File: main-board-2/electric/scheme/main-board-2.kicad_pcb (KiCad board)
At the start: 2 copper layers, 85 x 56 mm, 125 parts, among them K1 power-switch, K2 usb-power-switch, P1 batt, P10 rst, P11 screw-1, P13 screw-2, P14 gpio-big, P15 gpio-small, P16 moto-1, P17 moto-2, P2 CONN_4, P3 trigger-btn, P4 CONN_3X2, P5 reg-short-to-gnd-1, P6 reg-short-to-gnd-2, P7 bootloader, P8 cross board conn, P9 rst, Q1 IRLML2244, Q10 IRLML2244, Q11 sot223, Q12 bc857, Q13 irlml2244, Q2 BC847, Q3 IRLML2244, Q4 IRLML2244, Q5 BC847, Q6 BC847, Q7 BC847, Q8 BC847, Q9 IRLML2244, U1 LM317AEMP, U2 LM317AT, U3 LM317AEMP, U4 LM317AT, U5 LM293, U6 L298, U7 MINI-USB-B, X1 8MHz

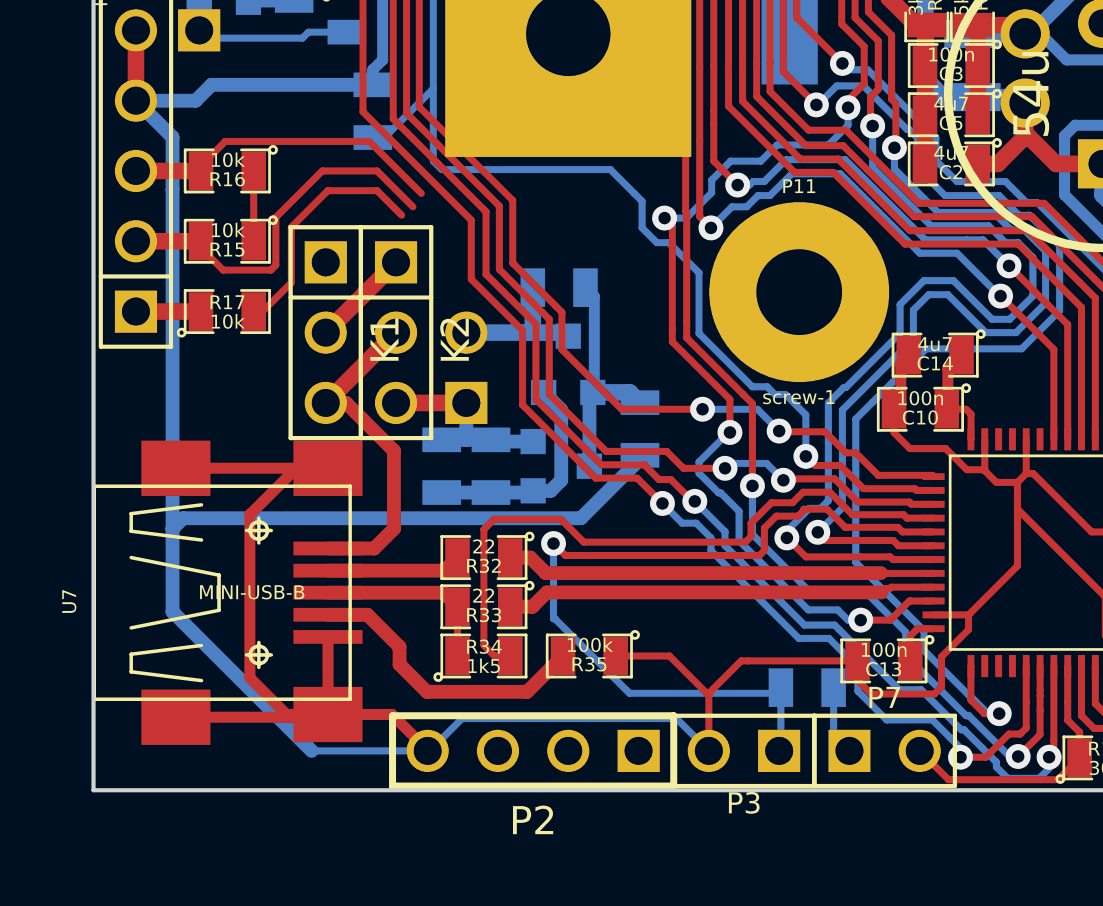
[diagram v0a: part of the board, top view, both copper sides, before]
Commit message: Routing...
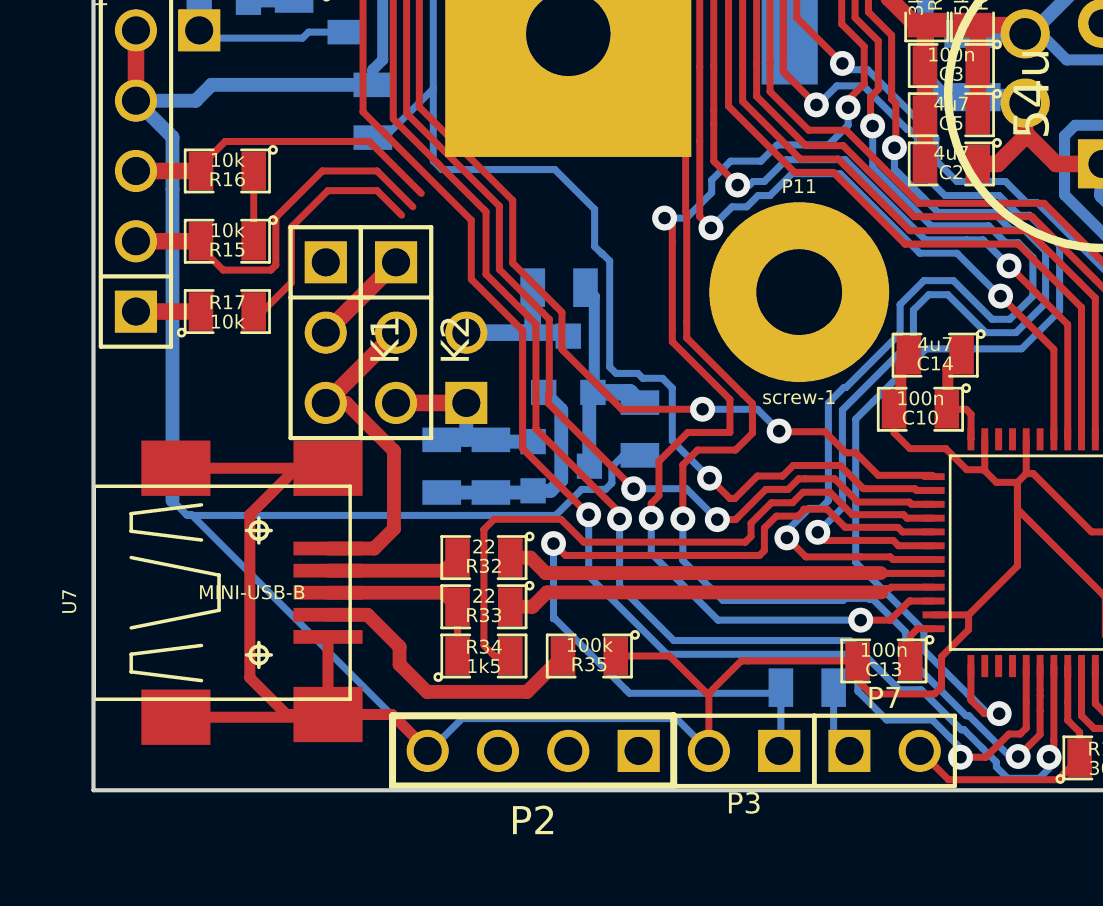
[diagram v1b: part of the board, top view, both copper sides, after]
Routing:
- net /scl-rpi: track 71.5 -> 76.5 mm
- net /swd-io: track 63.1 -> 67.5 mm
- net GND: track 433.4 -> 430.6 mm
- net /addon-pwr-en: track 45.8 -> 48.2 mm
- net /rpi-pwr-en: track 47.0 -> 49.0 mm
- net /sda-rpi: track 75.6 -> 77.5 mm
- net /gpio-5: track 57.9 -> 59.1 mm
